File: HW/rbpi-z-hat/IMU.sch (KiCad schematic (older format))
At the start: 11 parts, among them U1 MPU-9250

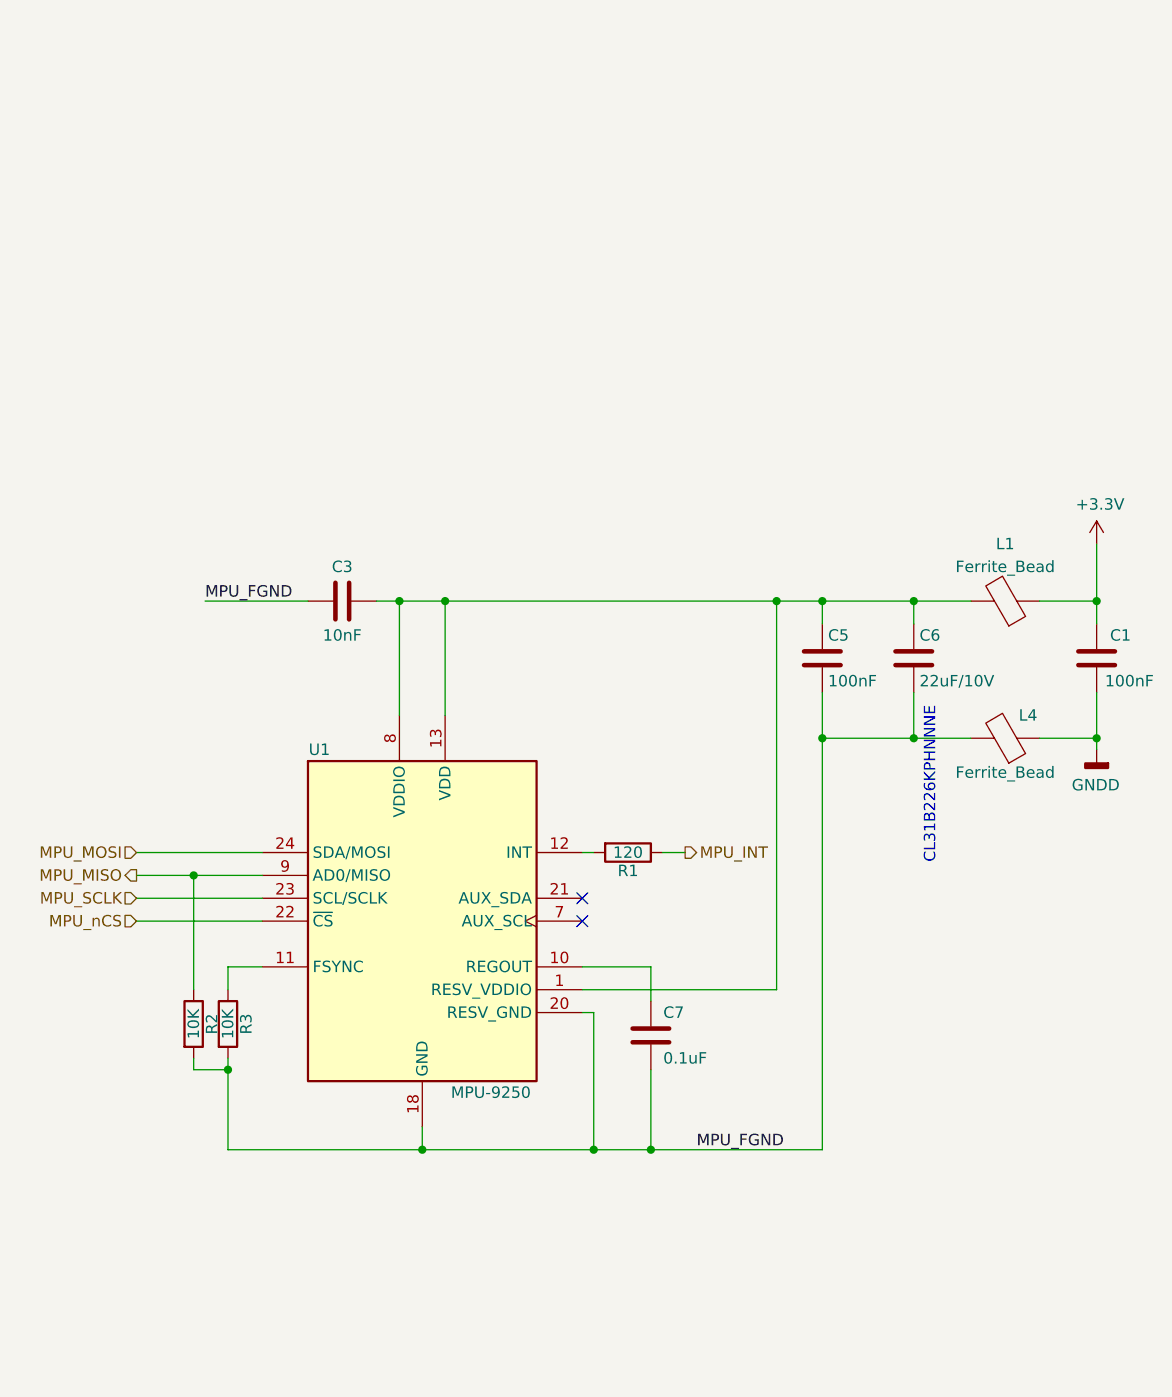
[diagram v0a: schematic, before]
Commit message: Commit...
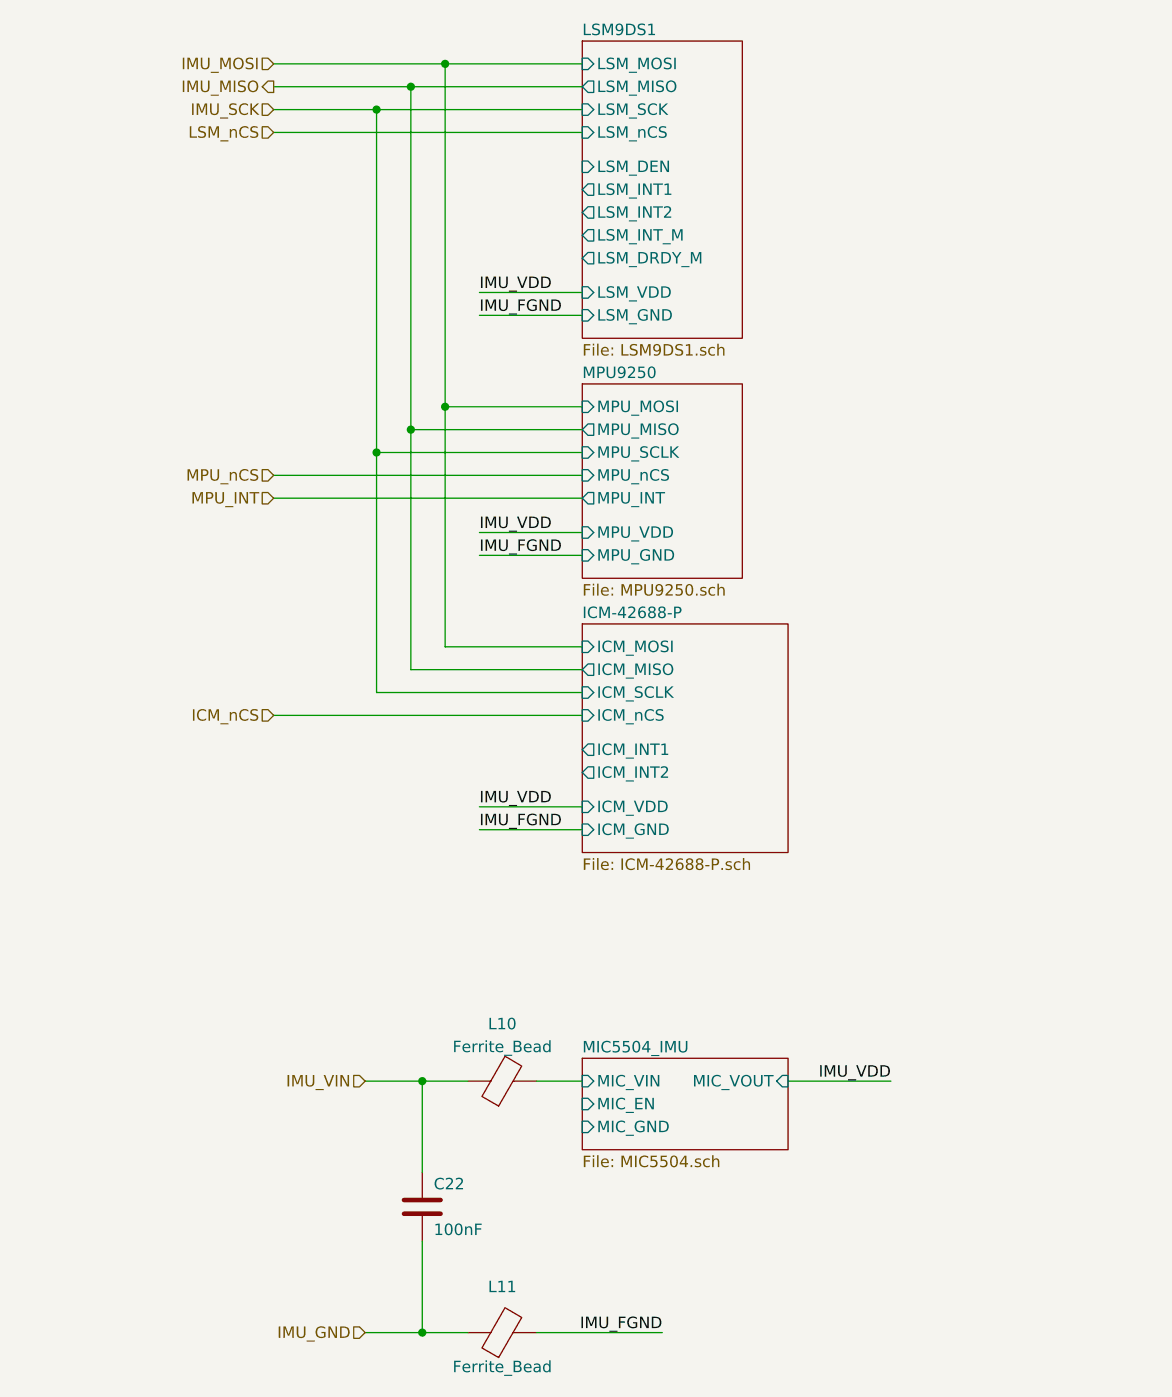
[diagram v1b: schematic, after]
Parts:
- removed C1, C5: 100nF, Capacitor_SMD:C_0603_1608Metric, symbol Device:C
- removed C3: 10nF, Capacitor_SMD:C_0603_1608Metric, symbol Device:C
- removed C6: 22uF/10V, Capacitor_SMD:C_1206_3216Metric, symbol Device:C
- removed C7: 0.1uF, Capacitor_SMD:C_0603_1608Metric, symbol Device:C
- removed L1, L4: Ferrite_Bead, Inductor_SMD:L_0603_1608Metric, symbol Device:Ferrite_Bead
- removed R1: 120, Resistor_SMD:R_0603_1608Metric, symbol Device:R
- removed R2, R3: 10K, Resistor_SMD:R_0603_1608Metric, symbol Device:R
- removed U1: MPU-9250, Package_DFN_QFN:QFN-24-1EP_3x3mm_P0.4mm_EP1.75x1.6mm, symbol Sensor_Motion:MPU-9250
- added C22: 100nF, Capacitor_SMD:C_0603_1608Metric, symbol Device:C
- added L10, L11: Ferrite_Bead, Inductor_SMD:L_0603_1608Metric, symbol Device:Ferrite_Bead
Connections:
- new net IMU_FGND: L11.2
- new net IMU_GND: C22.2, L11.1
- new net IMU_VIN: C22.1, L10.1
- new net MIC5504_IMU/MIC_VIN: L10.2
- no-connect marks 2 -> 0
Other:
- note removed: "CL31B226KPHNNNE"
